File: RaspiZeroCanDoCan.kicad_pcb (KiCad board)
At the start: 2 copper layers, 21 parts, among them IC1 MCP2562, P6 CAN_conn, P9 CAN_conn, U1 LD1117S50TR, U3 MCP2515-E/ST

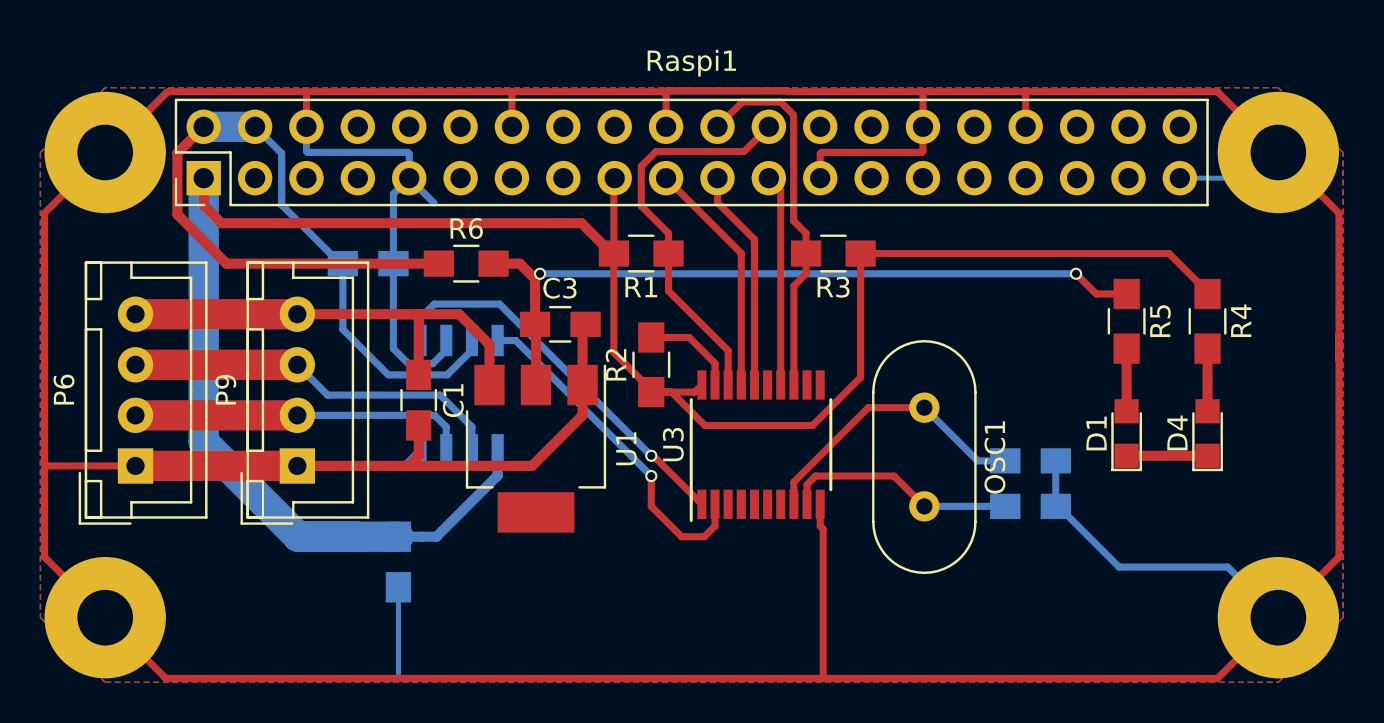
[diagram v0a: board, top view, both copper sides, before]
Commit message: update pcb
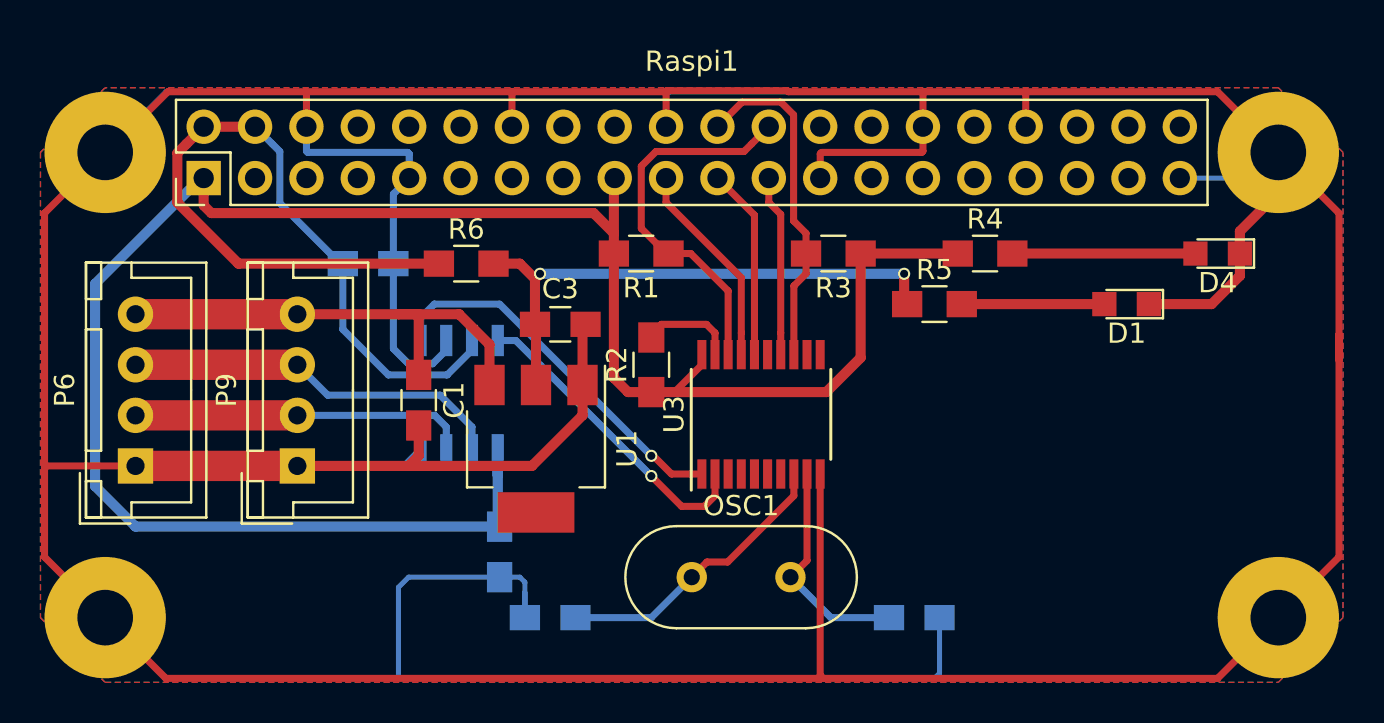
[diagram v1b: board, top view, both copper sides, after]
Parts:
- moved C2 25.0 mm to (141.5, 128.0), turned to 180 degrees
- moved OSC1 14.2 mm to (148.5, 126.0), turned to 0 degrees
- moved R4 11.5 mm to (163.0, 110.0), turned to 0 degrees
- moved R5 9.54 mm to (160.5, 112.5), turned to 0 degrees
- moved D4 8.91 mm to (174.5, 110.0), turned to 180 degrees
- moved C4 7.96 mm to (159.5, 128.0)
- moved D1 6.40 mm to (170.0, 112.5), turned to 180 degrees
- moved C5 5.02 mm to (139.0, 124.8)
- moved U3 1.50 mm to (151.9, 118.0)
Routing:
- net CAN_5V: track 37.4 -> 27.5 mm
- net +3V3: track 108.8 -> 102.4 mm
- net Net-(D4-Pad2): track 3.10 -> 9.05 mm
- net GND: track 471.0 -> 476.4 mm
- net Net-(D1-Pad2): track 3.10 -> 7.05 mm
- net CAN_RX: track 17.4 -> 15.9 mm
- net SPI_MISO: track 11.0 -> 9.49 mm
- net INT: track 18.4 -> 16.9 mm
- net SPI_CLK: track 10.5 -> 8.97 mm
- net SPI_MOSI: track 11.8 -> 10.3 mm
- net SPI_CS0: track 19.7 -> 19.0 mm
- net CAN_TX: track 19.4 -> 18.8 mm
